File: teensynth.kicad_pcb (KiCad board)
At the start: 2 copper layers, 89 parts, among them CON1 SJ-3523-SMT-TR, CON2 SJ-3523-SMT-TR, J1 Control_0, J10 LED_3_O, J11 LED_3_I, J12 LED_0_I, J13 LED_2_O, J14 Control_2, J15 Control_6, J16 LED_2_I, J17 LED_X_O, J18 LED_1_O, J19 LED_X_I, J2 Control_4, J20 Control_3, J21 Control_7, J22 LED_1_I, J23 LED_0_O, J24 10118193-0001LF, J25 10118193-0001LF, J3 LED_4_O, J4 LED_5_0, J5 LED_5_I, J6 LED_4_I, J7 Control_1, J8 Control_5, J9 LED_6_I, U1 CD74HC4051E, U2 MCP23017-E_SP, U3 Teensy3.2

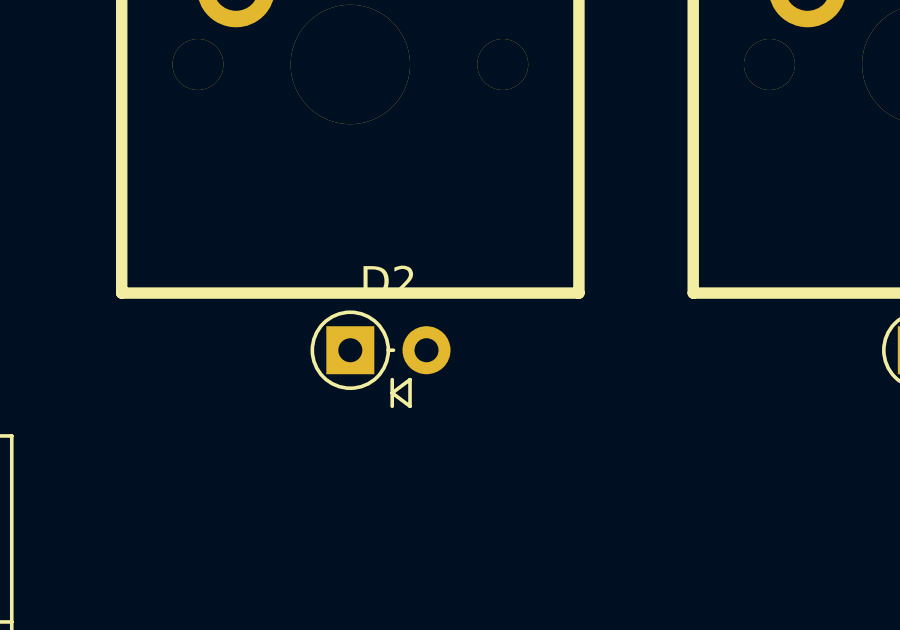
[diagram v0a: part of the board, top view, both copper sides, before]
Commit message: Update design rules
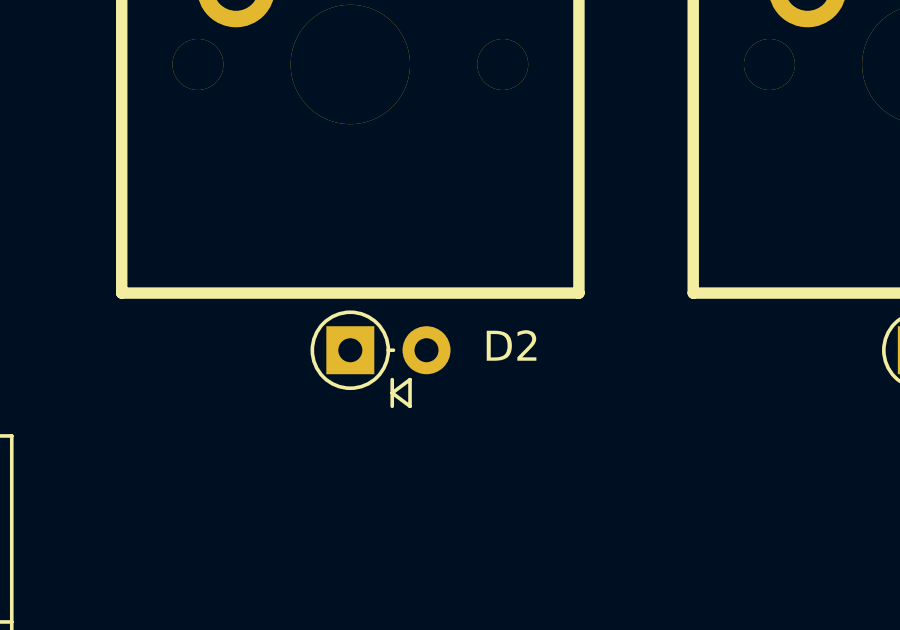
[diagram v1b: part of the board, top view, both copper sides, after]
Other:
- net class Default: trace_width 0.25 -> 0.2; via_dia 0.8 -> 0.6; via_drill 0.4 -> 0.3
- net class Power added: clearance 0.2, trace_width 0.7, via_dia 1, via_drill 0.5
- net class Test removed
- rule via_min_size: 0.4 -> 0.6
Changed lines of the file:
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@@
   )
   (setup
-    (last_trace_width 0.25)
+    (last_trace_width 0.2)
     (trace_clearance 0.2)
     (zone_clearance 0.508)
@@
     (segment_width 0.2)
     (edge_width 0.1)
-    (via_size 0.8)
-    (via_drill 0.4)
-    (via_min_size 0.4)
+    (via_size 0.6)
+    (via_drill 0.3)
+    (via_min_size 0.6)
     (via_min_drill 0.3)
-    (uvia_size 0.3)
-    (uvia_drill 0.1)
+    (uvia_size 0.6)
+    (uvia_drill 0.3)
     (uvias_allowed no)
     (uvia_min_size 0.2)
@@
     (solder_mask_min_width 0.25)
     (aux_axis_origin 0 0)
-    (visible_elements 7FFFF7FF)
+    (visible_elements 7FFFFFFF)
     (pcbplotparams
       (layerselection 0x010fc_ffffffff)
@@
   (net_class Default "This is the default net class."
     (clearance 0.2)
-    (trace_width 0.25)
-    (via_dia 0.8)
-    (via_drill 0.4)
-    (uvia_dia 0.3)
-    (uvia_drill 0.1)
-    (add_net +3V3)
-    (add_net +5V)
+    (trace_width 0.2)
+    (via_dia 0.6)
+    (via_drill 0.3)
+    (uvia_dia 0.6)
+    (uvia_drill 0.3)
     (add_net /A2)
     (add_net /Col0)
@@
     (add_net /SCL)
     (add_net /SDA)
-    (add_net GND)
     (add_net "Net-(CON1-Pad1)")
     (add_net "Net-(CON1-Pad2)")
@@
     (add_net "Net-(U3-Pad9)")
   )
-  (net_class Test ""
+  (net_class Power ""
     (clearance 0.2)
-    (trace_width 0.38)
-    (via_dia 0.8)
-    (via_drill 0.4)
-    (uvia_dia 0.3)
-    (uvia_drill 0.1)
+    (trace_width 0.7)
+    (via_dia 1)
+    (via_drill 0.5)
+    (uvia_dia 1)
+    (uvia_drill 0.5)
+    (add_net +3V3)
+    (add_net +5V)
+    (add_net GND)
   )
   (module digikey-footprints:Switch_Slide_11.6x4mm_SJ-3523-SMT (layer F.Cu)
@@
     (descr "D, DO-35_SOD27 series, Axial, Vertical, pin pitch=2.54mm, , length*diameter=4*2mm^2, , http://www.diodes.com/_files/packages/DO-35.pdf")
     (tags "D DO-35_SOD27 series Axial Vertical pin pitch 2.54mm  length 4mm diameter 2mm")
-    (fp_text reference D2 (at 1.27 -2.266371) (layer F.SilkS)
-      (effects (font (size 1 1) (thickness 0.15)))
-    )
+    (fp_text reference D2 (at 5.375 -0.1125) (layer F.SilkS)
+      (effects (font (size 1 1) (thickness 0.15)))
+    )

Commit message: Wire up the matrix to the io expander
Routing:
- net /Row0: track 0.00 -> 282.9 mm, vias 0 -> 1
- net /Row1: track 0.00 -> 276.0 mm, vias 0 -> 1
- net /ColD: track 0.00 -> 194.4 mm
- net /Col0: track 0.00 -> 172.8 mm
- net /ColC: track 0.00 -> 165.4 mm
- net /Col1: track 0.00 -> 159.4 mm
- net /ColB: track 0.00 -> 147.8 mm
- net /ColA: track 0.00 -> 129.3 mm
- net /Col2: track 0.00 -> 124.4 mm
- net /Col3: track 0.00 -> 121.3 mm
- net /Col4: track 0.00 -> 102.4 mm
- net /Col9: track 0.00 -> 96.5 mm
- net /Col8: track 0.00 -> 87.6 mm
- net /Col5: track 0.00 -> 83.6 mm
- net /Col7: track 0.00 -> 62.6 mm
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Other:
- net class Default: trace_width 0.2 -> 0.4; via_dia 0.6 -> 1; via_drill 0.3 -> 0.5
- net class Power: trace_width 0.7 -> 1
